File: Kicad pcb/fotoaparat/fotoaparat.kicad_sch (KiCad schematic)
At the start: 72 parts, among them IC1 Lineární Regulátor, IC3 Lineární Regulátor Displaye, J1 USB Konektor, J2 SWD, J3 LCD konektor, J4 Baterie, J5 GSD090012SEU, J6 UART, J7 Kamera, J9 Conn_01x11_Socket, U1 STM32L496RETx, U2 MCP73833-FCI/UN, Y1 8mhz krystal

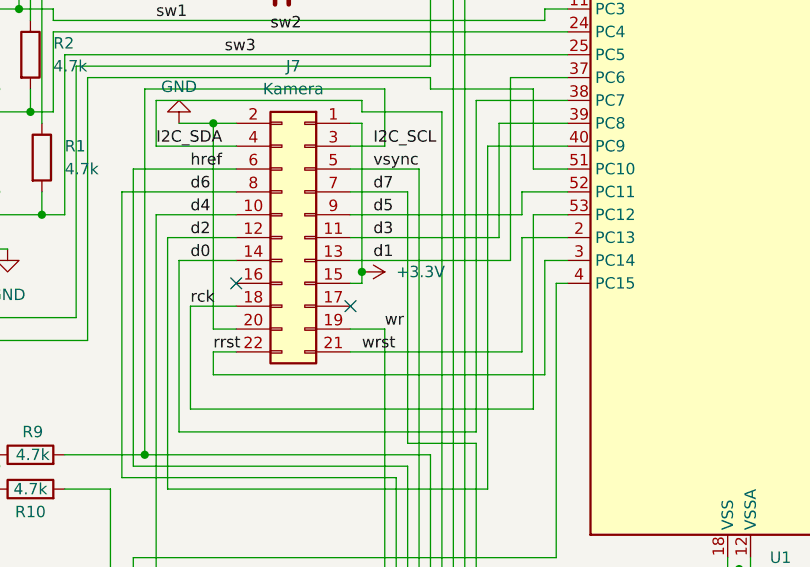
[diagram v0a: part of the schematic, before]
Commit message: Připraveno na výrobu
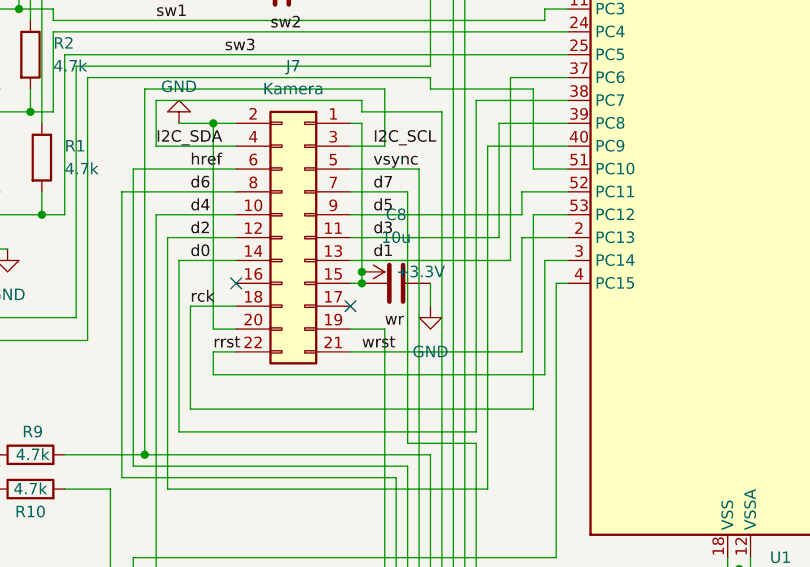
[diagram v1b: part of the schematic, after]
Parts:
- added C8: 10u, Capacitor_THT:CP_Radial_D5.0mm_P2.50mm, symbol Device:C
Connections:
- net +3.3V: now also C8.1
- net GND: now also C8.2
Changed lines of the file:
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@@
 	)
 	(junction
+		(at 106.68 109.22)
+		(diameter 0)
+		(color 0 0 0 0)
+	)
+	(junction
 		(at 213.36 59.69)
 		(diameter 0)
@@
 	(wire
 		(pts
+			(xy 114.3 109.22) (xy 114.3 111.76)
+		)
+		(stroke
+			(width 0)
+			(type default)
+		)
+	)
+	(wire
+		(pts
 			(xy 207.01 20.32) (xy 207.01 19.05)
 		)
@@
 	(symbol
 		(lib_id "Device:C")
+		(at 110.49 109.22 90)
+		(unit 1)
+		(exclude_from_sim no)
+		(in_bom yes)
+		(on_board yes)
+		(dnp no)
+		(fields_autoplaced yes)
+		(property "Reference" "C8"
+			(at 110.49 101.6 90)
+			(effects
+				(font
+					(size 1.27 1.27)
+				)
+			)
+		)
+		(property "Value" "10u"
+			(at 110.49 104.14 90)
+			(effects
+				(font
+					(size 1.27 1.27)
+				)
+			)
+		)
+		(property "Footprint" "Capacitor_THT:CP_Radial_D5.0mm_P2.50mm"
+			(at 114.3 108.2548 0)
+			(effects
+				(font
+					(size 1.27 1.27)
+				)
+				(hide yes)
+			)
+		)
+		(property "Datasheet" "~"
+			(at 110.49 109.22 0)
+			(effects
+				(font
+					(size 1.27 1.27)
+				)
+				(hide yes)
+			)
+		)
+		(property "Description" "Unpolarized capacitor"
+			(at 110.49 109.22 0)
+			(effects
+				(font
+					(size 1.27 1.27)
+				)
+				(hide yes)
+			)
+		)
+		(pin "1"
+		)
+		(pin "2"
+		)
+		(instances
+			(project ""
+				(path "/af31909f-b2e8-4f24-bd61-08599f2fc290"
+					(reference "C8")
+					(unit 1)
+				)
+			)
+		)
+	)
+	(symbol
+		(lib_id "Device:C")
 		(at -77.47 172.72 270)
 		(unit 1)
@@
 					(unit 1)
 				)
+			)
+		)
+	)
+	(symbol
+		(lib_id "power:GND")
+		(at 114.3 111.76 0)
+		(unit 1)
+		(exclude_from_sim no)
+		(in_bom yes)
+		(on_board yes)
+		(dnp no)
+		(fields_autoplaced yes)
+		(property "Reference" "#PWR050"
+			(at 114.3 118.11 0)
+			(effects
+				(font
+					(size 1.27 1.27)
+				)
+				(hide yes)
+			)
+		)
+		(property "Value" "GND"
+			(at 114.3 116.84 0)
+			(effects
+				(font
+					(size 1.27 1.27)
+				)
+			)
+		)
+		(property "Footprint" ""
+			(at 114.3 111.76 0)
+			(effects
+				(font
+					(size 1.27 1.27)
+				)
+				(hide yes)
+			)
+		)
+		(property "Datasheet" ""
+			(at 114.3 111.76 0)
+			(effects
+				(font
+					(size 1.27 1.27)
+				)
+				(hide yes)
+			)
+		)
+		(property "Description" "Power symbol creates a global label with name \"GND\" , ground"
+			(at 114.3 111.76 0)
+			(effects
+				(font
+					(size 1.27 1.27)
+				)
+				(hide yes)
+			)
+		)
+		(pin "1"
+		)
+		(instances
+			(project ""
+				(path "/af31909f-b2e8-4f24-bd61-08599f2fc290"
+					(reference "#PWR050")
+					(unit 1)
+				)

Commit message: Úprava designu
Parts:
- removed C10, C11, C12, C14, C21, C9: 100n, Capacitor_SMD:C_0805_2012Metric_Pad1.18x1.45mm_HandSolder, symbol Device:C
- removed C15, C16, C22: 1u, Capacitor_SMD:C_0805_2012Metric_Pad1.18x1.45mm_HandSolder, symbol Device:C
- removed C17, C18: 30p, Capacitor_SMD:C_0805_2012Metric_Pad1.18x1.45mm_HandSolder, symbol Device:C
- removed C7, C8: 10u, Capacitor_THT:CP_Radial_D5.0mm_P2.50mm, symbol Device:C
- removed D1, D2, D3: LED, LED_SMD:LED_0805_2012Metric_Pad1.15x1.40mm_HandSolder, symbol Device:LED
- removed FB1: 120R, Inductor_SMD:L_0805_2012Metric_Pad1.05x1.20mm_HandSolder, symbol Device:FerriteBead
- removed H1, H2, H3, H4: MountingHole, MountingHole:MountingHole_3.2mm_M3, symbol Mechanical:MountingHole
- removed IC1: Lineární Regulátor, Package_TO_SOT_SMD:TSOT-23-5_HandSoldering, symbol NCP718ASN330T1G:NCP718ASN330T1G
- removed IC3: Lineární Regulátor Displaye, Package_TO_SOT_SMD:TSOT-23-5_HandSoldering, symbol NCP718ASN330T1G:NCP718ASN330T1G
- removed J1: USB Konektor, 47436:473460001, symbol 47346-0001:47346-0001
- removed J2: SWD, Connector_PinHeader_2.54mm:PinHeader_1x04_P2.54mm_Vertical, symbol Connector:Conn_01x04_Socket
- removed J3: LCD konektor, FFC2A32-20-T:GCT_FFC2A32-20-T, symbol FFC2A32-20-T:FFC2A32-20-T
- removed J4: Baterie, Connector_PinSocket_2.54mm:PinSocket_1x02_P2.54mm_Horizontal, symbol Connector:Conn_01x02_Socket
- removed J5: GSD090012SEU, gsd09:GSD090012SEU_AMP, symbol 2025-09-30_19-14-30:GSD090012SEU
- removed J6: UART, Connector_PinHeader_2.54mm:PinHeader_1x02_P2.54mm_Vertical, symbol Connector:Conn_01x02_Socket
- removed J7: Kamera, Connector_PinSocket_2.54mm:PinSocket_2x11_P2.54mm_Vertical, symbol Connector_Generic:Conn_02x11_Odd_Even
- removed J9: Conn_01x11_Socket, Connector_PinSocket_2.54mm:PinSocket_1x11_P2.54mm_Horizontal, symbol Connector:Conn_01x11_Socket
- removed R10, R11, R12, R13, R14, R15, R16, R17, R18, R19, R20, R21, R22, R23, R24, R26, R9: 4.7k, Resistor_SMD:R_0805_2012Metric_Pad1.20x1.40mm_HandSolder, symbol Device:R
- removed R25, R7: 1k, Resistor_SMD:R_0805_2012Metric_Pad1.20x1.40mm_HandSolder, symbol Device:R
- removed R8: 2, Resistor_SMD:R_0805_2012Metric_Pad1.20x1.40mm_HandSolder, symbol Device:R
- removed S1: Zapínací spínač, mfs:MFS201N24Z, symbol MFS201N-24-Z:MFS201N-24-Z
- removed S2: tlačítko doleva, mc3:MC32829, symbol MC32829:MC32829
- removed S3: prostřední tlačítko, mc3:MC32829, symbol MC32829:MC32829
- removed S4: tlačítko doprava, mc3:MC32829, symbol MC32829:MC32829
- removed S5: spínač, cfs201mb:CFS0201MB, symbol CFS-0201MB:CFS-0201MB
- removed TH1: 10k, Connector_PinSocket_2.54mm:PinSocket_1x02_P2.54mm_Horizontal, symbol Device:Thermistor
- removed U1: STM32L496RETx, Package_QFP:LQFP-64_10x10mm_P0.5mm, symbol MCU_ST_STM32L4:STM32L496RETx
- removed U2: MCP73833-FCI/UN, MCP:MSOP10_MC_MCH, symbol 2025-09-30_17-20-56:MCP73833-FCI_UN
- removed Y1: 8mhz krystal, hc4:HC49S830507030ATF, symbol HC49S-8-30-50-70-30-ATF:HC49S-8-30-50-70-30-ATF
- added J1: Conn_02x01, Connector_PinHeader_2.54mm:PinHeader_2x01_P2.54mm_Vertical, symbol Connector_Generic:Conn_02x01
- added Q1, Q2: BC547, Package_TO_SOT_THT:TO-92_Inline, symbol Transistor_BJT:BC547
- added SW1: SW_Push_Dual, Tlačítko:tlačítko 6x6x12, symbol Switch:SW_Push_Dual
- added U1: TP4056, TP4056:TP4056, symbol tp4056:tp4056
- added U2: ov7670 fifo, ov7670:ov7670, symbol ov7670:ov7670
- added U3: Stm32 Bluepill, Stm32 Bluepill:Bluepill, symbol Stm32 Bluepill:Stm32_Bluepill
- added U4: Lcd Display, Lcd Display:ili9341, symbol ili9341:lcd_ili9341
- added U5: FJ08k, Tlačítko:FJ08K-S, symbol Joystick FJ08K:FJ08k
- added U6, U8, U9: Me6211c, Package_TO_SOT_SMD:SOT-23-5, symbol Me6211c:Me6211c
- added U7: VBsemi SI2312CDS-T1-GE3, Package_TO_SOT_SMD:SOT-23W_Handsoldering, symbol Mosfet N:Mosfet_N
- BZ1: footprint Inductor_SMD:L_SXN_SMDRI73 -> Jiangsu:Jiangsu
- C1, C2, C3, C4, C5, C6: value 1u -> 4.7uf
- R1, R2: value 4.7k -> 100k; footprint Resistor_SMD:R_0805_2012Metric_Pad1.20x1.40mm_HandSolder -> Resistor_THT:R_Axial_DIN0207_L6.3mm_D2.5mm_P10.16mm_Horizontal
- R3: value 4.7k -> 10k; footprint Resistor_SMD:R_0805_2012Metric_Pad1.20x1.40mm_HandSolder -> Resistor_THT:R_Axial_DIN0207_L6.3mm_D2.5mm_P10.16mm_Horizontal
- R4: value 1k -> 100k; footprint Resistor_SMD:R_0805_2012Metric_Pad1.20x1.40mm_HandSolder -> Resistor_THT:R_Axial_DIN0207_L6.3mm_D2.5mm_P10.16mm_Horizontal
- R5: value 1k -> 30k; footprint Resistor_SMD:R_0805_2012Metric_Pad1.20x1.40mm_HandSolder -> Resistor_THT:R_Axial_DIN0207_L6.3mm_D2.5mm_P10.16mm_Horizontal
- R6: value 1k -> 50k; footprint Resistor_SMD:R_0805_2012Metric_Pad1.20x1.40mm_HandSolder -> Resistor_THT:R_Axial_DIN0207_L6.3mm_D2.5mm_P10.16mm_Horizontal
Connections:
- net +3.3V LCD is gone; now on net GND: C6.2
- net buzzer is gone; now on net +BATT: BZ1.1 (+)
- net sw2 is gone; now on an unnamed net: R2.2
- net +3.3V: now also C2.1, SW1.2, U3.23 (3v3), U5.1 (Y1), U5.4 (X1), U6.5 (Vout); no longer C4.2, R1.1, R2.1, R3.1
- net +BATT: now also R5.2, U1.5 (Bat+); no longer C2.1, C3.1, C5.1
- net GND: now also C4.2, R2.1, R3.1, R4.1, Q1.3 (E), Q2.3 (E), U1.4 (OUT-), U2.2 (gnd), U2.20 (oe), U3.19 (gnd), U3.21 (gnd), U3.22 (gnd), U4.13 (gnd), U5.2 (gnd), U5.5 (gnd), U6.2 (Vss), U6.4 (NC), U8.2 (Vss), U8.4 (NC), U9.2 (Vss), U9.4 (NC); no longer BZ1.2 (-), C4.1, C6.1
- net at R5.1: now also R4.2, U3.35 (pa1)
- net at R6.2: now also U3.9 (pa12)
- net Indikátor Nabíjení: no longer names the net of R6.1
- net Indikátor Nabíjení: now also Q1.2 (B), SW1.3
- net VBUS renamed +4V
- net +4V: now also C3.1, C5.1, U6.1 (Vin), U6.3 (CE), U7.3 (Drain), U8.1 (Vin), U8.3 (CE), U9.1 (Vin), U9.3 (CE)
- net sw1 renamed tx
- net tx: now also J1.1 (Pin_1), SW1.1, U3.6 (pa9)
- net sw3: no longer names the net of R1.2
- net sw3: now also SW1.4, U1.3 (OUT+), U7.2 (Source_gnd)
- new net: BZ1.2 (-), Q2.1 (C)
- new net: Q2.2 (B), U3.5 (pa8)
- new net: U3.28 (pb0), U4.10 (Dc)
- new net: U3.27 (pb1), U4.11 (Reset)
- new net: U3.32 (pa4), U4.12 (Cs)
- new net: U3.31 (pa5), U4.15 (sd_sck), U4.5 (T_clk), U4.8 (sck)
- new net: U3.30 (pa6), U4.16 (sd_miso), U4.2 (T_do), U4.6 (Sdo_miso)
- new net: U3.29 (pa7), U4.17 (sd_mosi), U4.3 (T_Din), U4.9 (sdi_mosi)
- new net: U3.1 (pb12), U4.18 (sd_cs)
- new net: U3.8 (pa11), U4.4 (T_cs)
- new net: U2.19 (wr), U3.10 (pa15)
- new net: U2.7 (d7), U3.11 (pb3)
- new net: U2.9 (d5), U3.12 (pb4)
- new net: U2.11 (d3), U3.13 (pb5)
- new net: U2.3 (sioc), U3.14 (pb6)
- new net: U2.4 (siod), U3.15 (pb7)
- new net: U2.13 (d1), U3.16 (pb8)
- new net: U2.8 (d6), U3.17 (pb9)
- new net: U2.14 (d0), U3.2 (pb13)
- new net: U2.10 (d4), U3.25 (pb11)
- new net: U2.12 (d2), U3.26 (pb10)
- new net: U2.18 (rck), U3.3 (pb14)
- new net: U3.33 (pa3), U5.6 (X2)
- new net: U3.34 (pa2), U5.3 (Y2)
- new net: U2.5 (vsync), U3.36 (pa0)
- new net: U2.22 (rrst), U3.4 (pb15)
- new net: Q1.1 (C), R1.1, U7.1 (Gate)
- new net +3.3V lcd: C6.1, U4.14 (Vcc), U4.7 (Led_3.3v), U9.5 (Vout)
- new net +3.3V ov7670: C4.1, U2.1 (3v3), U2.15 (rst), U8.5 (Vout)
- new net +3V3: U3.20 (3v3)
- new net -BATT: U1.6 (Bat-)
- new net rx: J1.2 (Pin_2), U2.21 (wrst), U3.7 (pa10)
- no-connect marks 35 -> 14
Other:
- note removed: "Regulátory"
- note removed: "Stm32 mikrokontrolér"

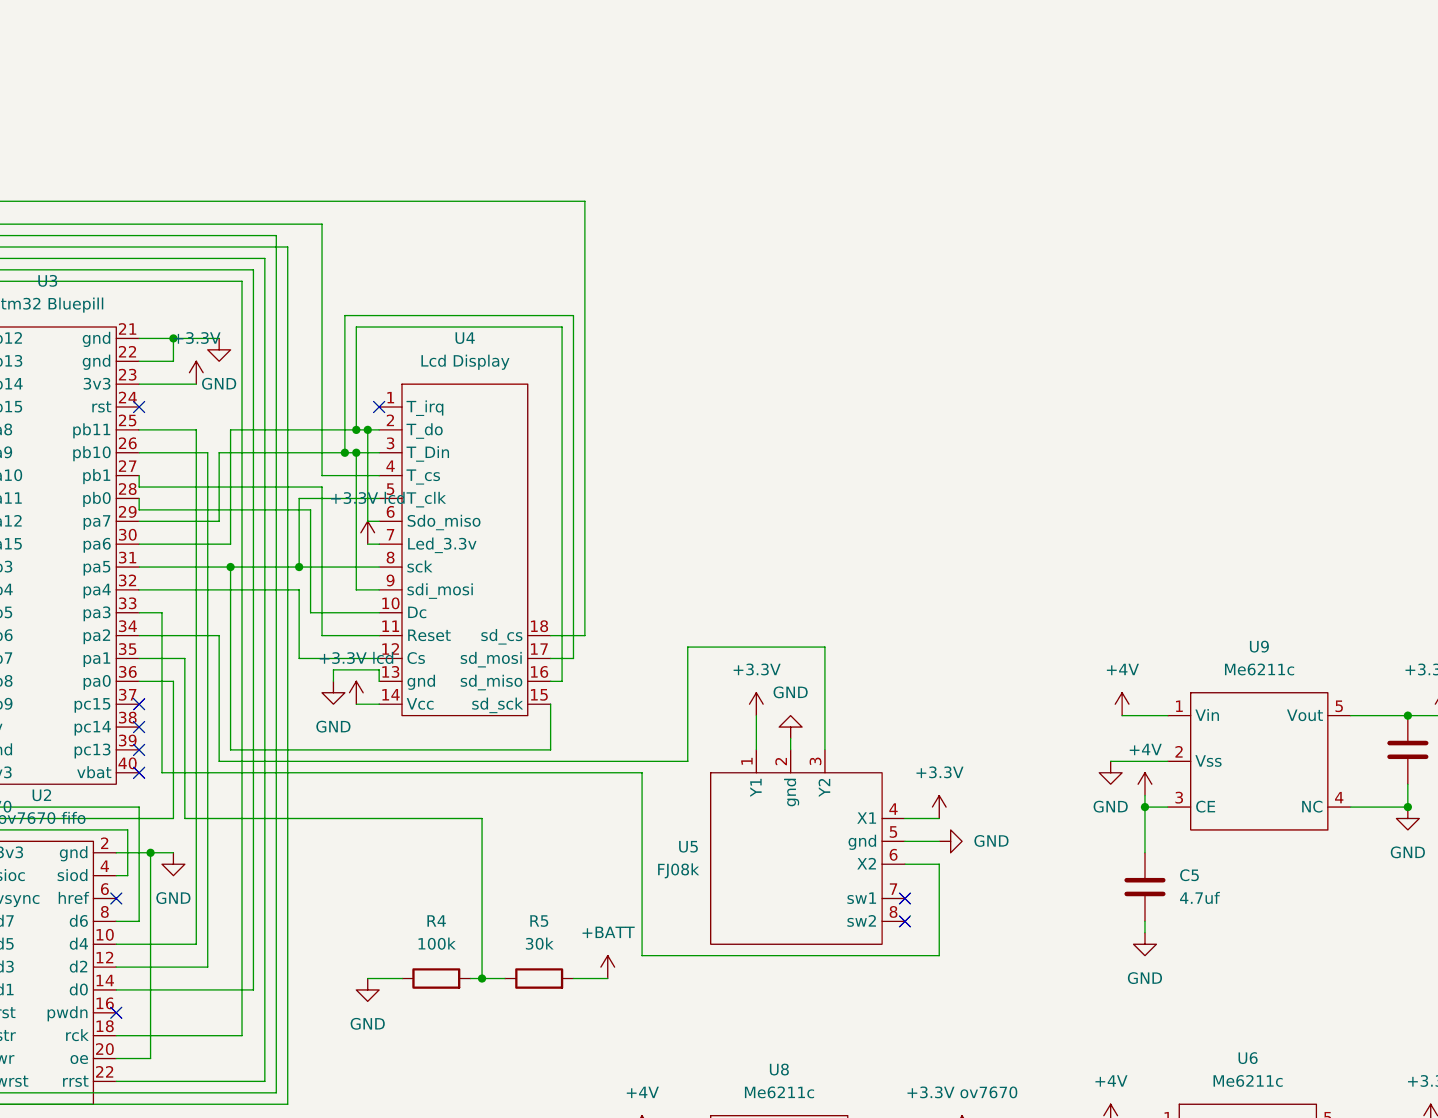
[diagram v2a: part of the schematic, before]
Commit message: Úprava designu
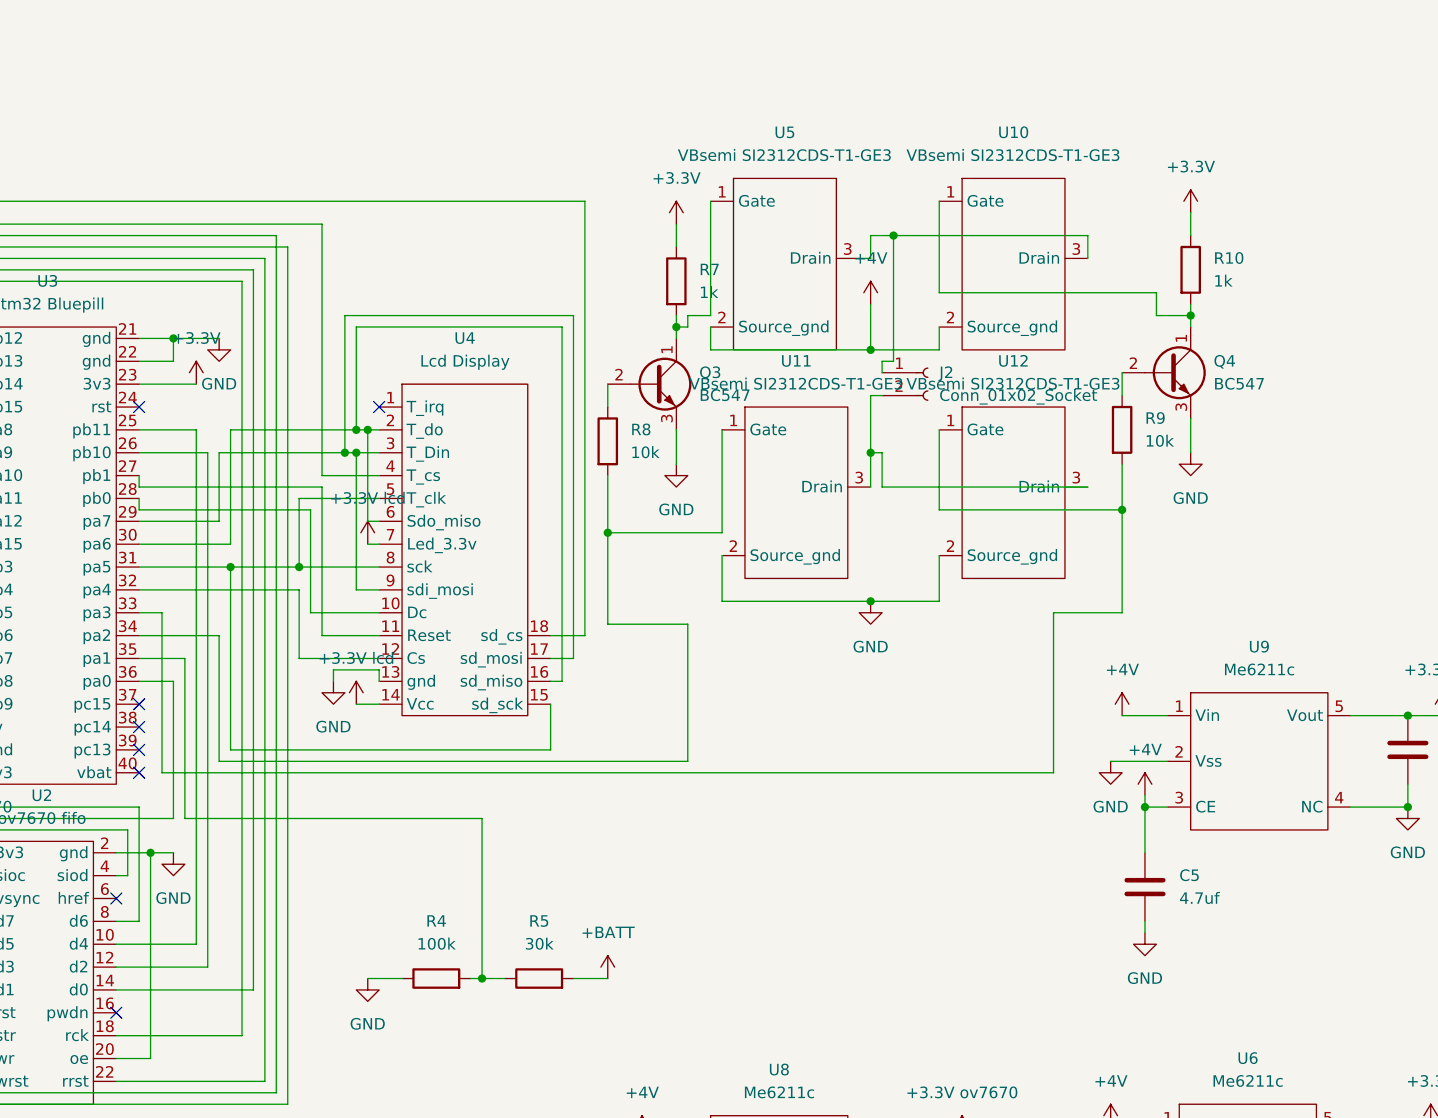
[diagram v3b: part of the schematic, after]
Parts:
- removed U5: FJ08k, Tlačítko:FJ08K-S, symbol Joystick FJ08K:FJ08k
- added J2: Conn_01x02_Socket, Connector_PinSocket_2.54mm:PinSocket_1x02_P2.54mm_Vertical, symbol Connector:Conn_01x02_Socket
- added Q3, Q4: BC547, Package_TO_SOT_THT:TO-92_Inline, symbol Transistor_BJT:BC547
- added R10, R7: 1k, Resistor_THT:R_Axial_DIN0207_L6.3mm_D2.5mm_P10.16mm_Horizontal, symbol Device:R
- added R8, R9: 10k, Resistor_THT:R_Axial_DIN0207_L6.3mm_D2.5mm_P10.16mm_Horizontal, symbol Device:R
- added U10, U11, U12, U5: VBsemi SI2312CDS-T1-GE3, Package_TO_SOT_SMD:SOT-23W_Handsoldering, symbol Mosfet N:Mosfet_N
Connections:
- net +3.3V: now also R10.1, R7.1
- net +4V: now also U10.2 (Source_gnd), U5.2 (Source_gnd)
- net GND: now also Q3.3 (E), Q4.3 (E), U11.2 (Source_gnd), U12.2 (Source_gnd)
- net at U3.33 (pa3): now also R9.2, U12.1 (Gate)
- net at U3.34 (pa2): now also R8.2, U11.1 (Gate)
- new net: Q4.1 (C), R10.2, U10.1 (Gate)
- new net: Q3.2 (B), R8.1
- new net: J2.2 (Pin_2), U11.3 (Drain), U12.3 (Drain)
- new net: Q4.2 (B), R9.1
- new net: J2.1 (Pin_1), U10.3 (Drain), U5.3 (Drain)
- new net: Q3.1 (C), R7.2, U5.1 (Gate)
- no-connect marks 14 -> 12
